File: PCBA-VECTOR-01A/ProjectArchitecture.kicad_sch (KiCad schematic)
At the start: 4 parts, among them J10 Conn_02x06_Odd_Even, J11 Conn_02x06_Odd_Even, J12 Conn_02x06_Odd_Even, J9 Conn_02x06_Odd_Even

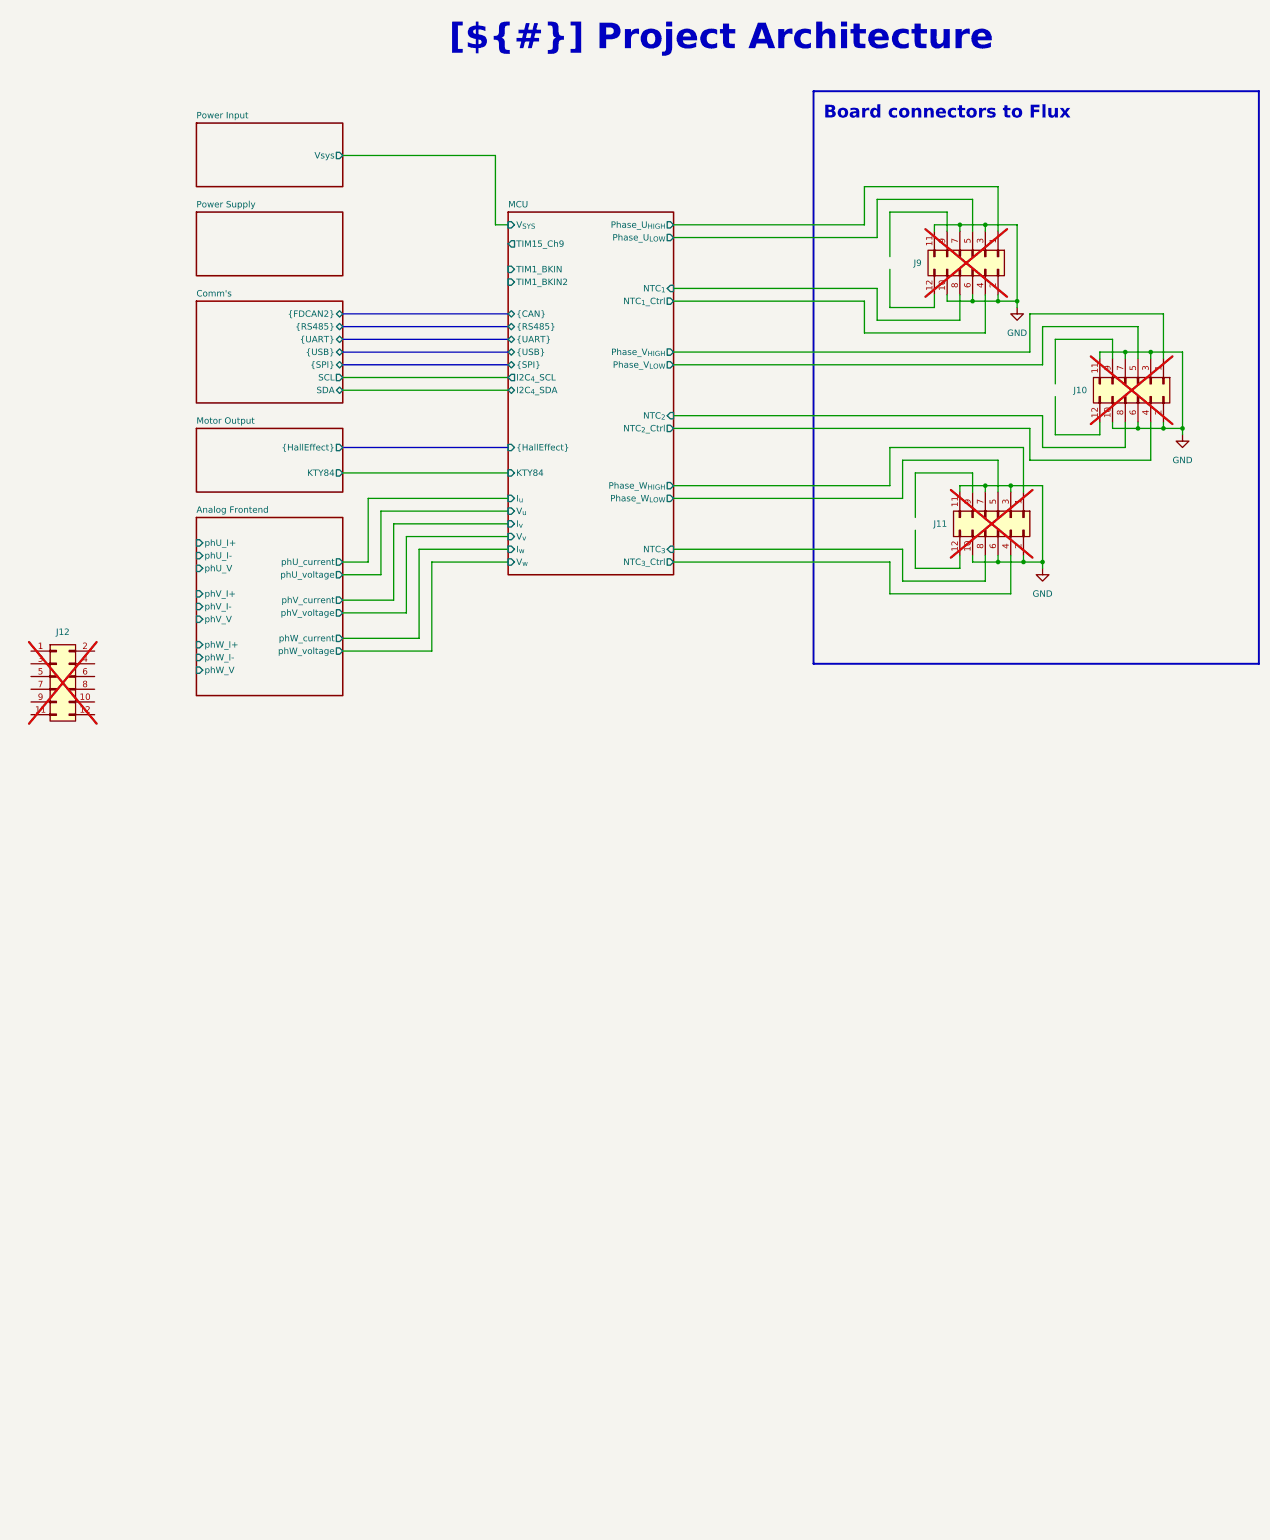
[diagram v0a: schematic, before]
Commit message: More routing on FLux
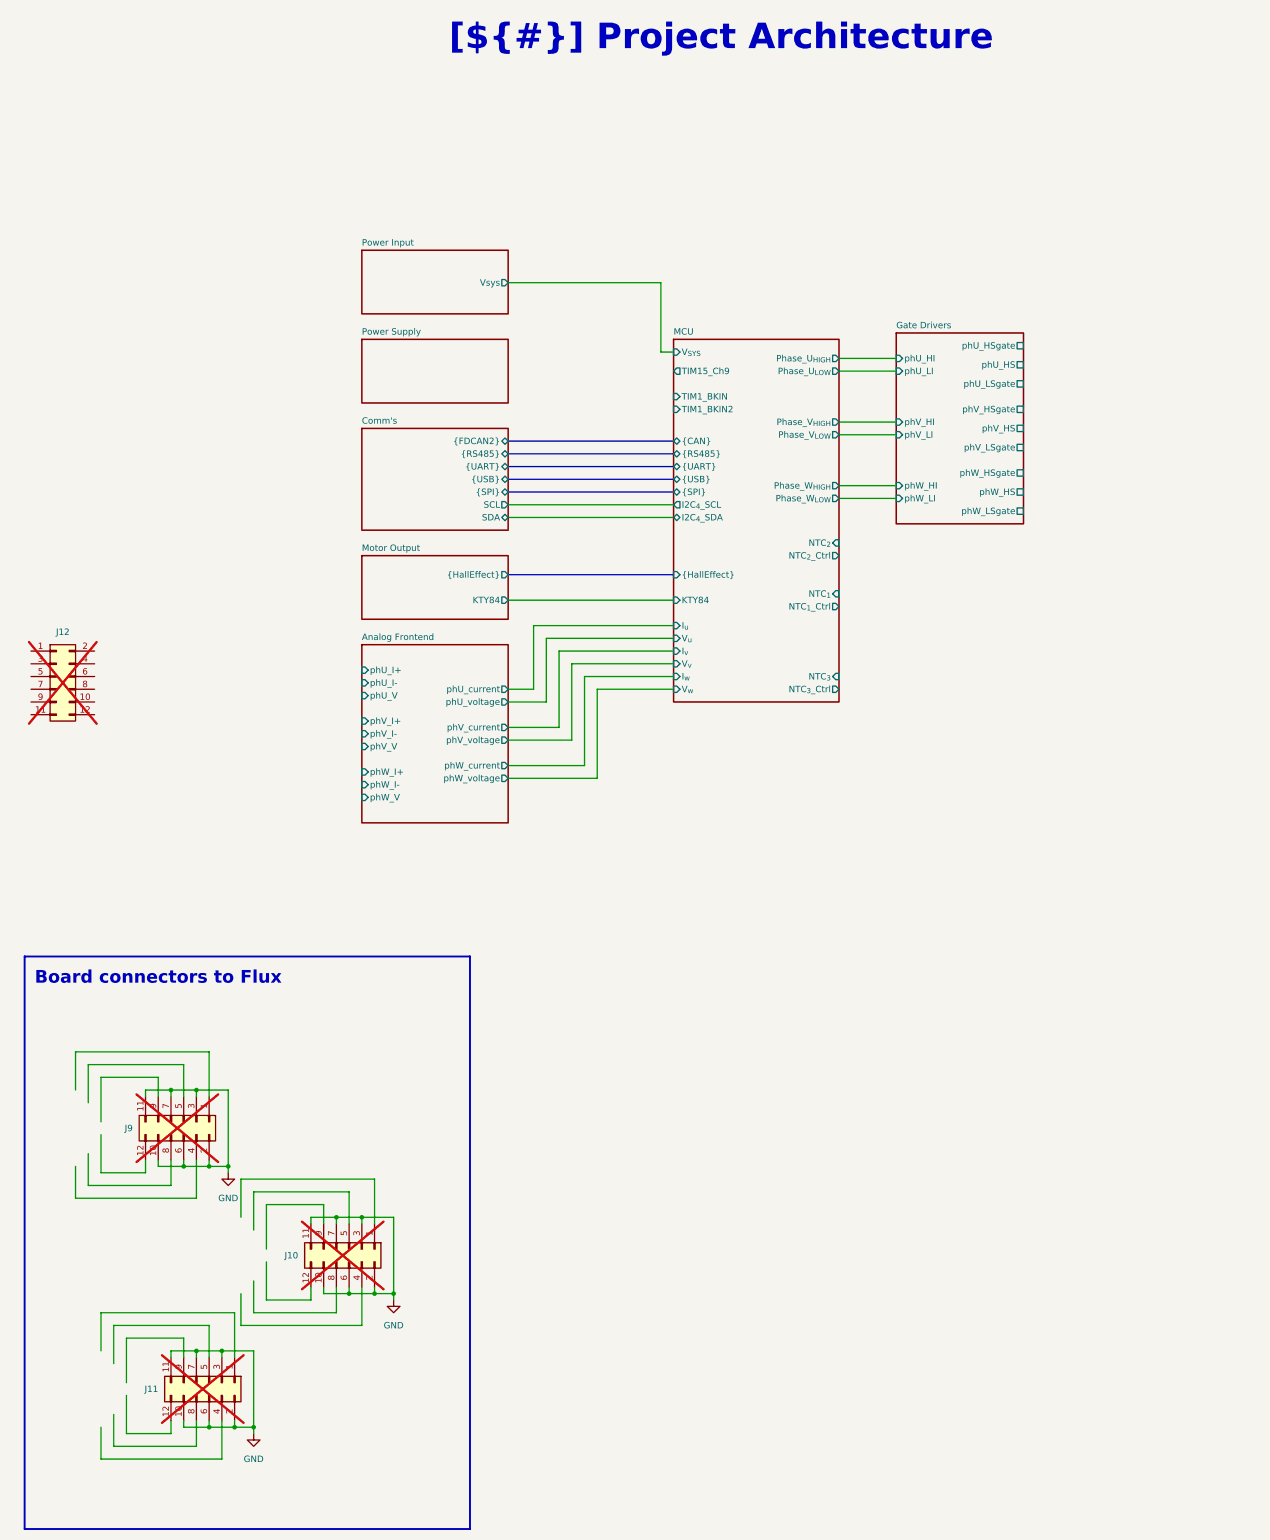
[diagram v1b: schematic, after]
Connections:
- net MCU/NTC_{1}: no longer J9.8 (Pin_8)
- net MCU/NTC_{1}_Ctrl: no longer J9.4 (Pin_4)
- net MCU/NTC_{2}: no longer J10.8 (Pin_8)
- net MCU/NTC_{2}_Ctrl: no longer J10.4 (Pin_4)
- net MCU/NTC_{3}: no longer J11.8 (Pin_8)
- net MCU/NTC_{3}_Ctrl: no longer J11.4 (Pin_4)
- net MCU/Phase_U_{HIGH}: no longer names the net of J9.1 (Pin_1)
- net MCU/Phase_U_{LOW}: no longer names the net of J9.5 (Pin_5)
- net MCU/Phase_V_{HIGH}: no longer names the net of J10.1 (Pin_1)
- net MCU/Phase_V_{LOW}: no longer names the net of J10.5 (Pin_5)
- net MCU/Phase_W_{HIGH}: no longer names the net of J11.1 (Pin_1)
- net MCU/Phase_W_{LOW}: no longer names the net of J11.5 (Pin_5)
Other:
- added sheet Gate Drivers (GateDrivers.kicad_sch)
- moved on the sheet: J10, J11, J9
